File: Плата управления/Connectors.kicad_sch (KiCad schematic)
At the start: 10 parts, among them J1 A, J2 B, J3 C, J4 Conn_01x10, J5 Conn_01x03_Pin, J6 Conn_01x02, J7 Conn_01x10, J8 Conn_01x02, J9 Conn_01x04

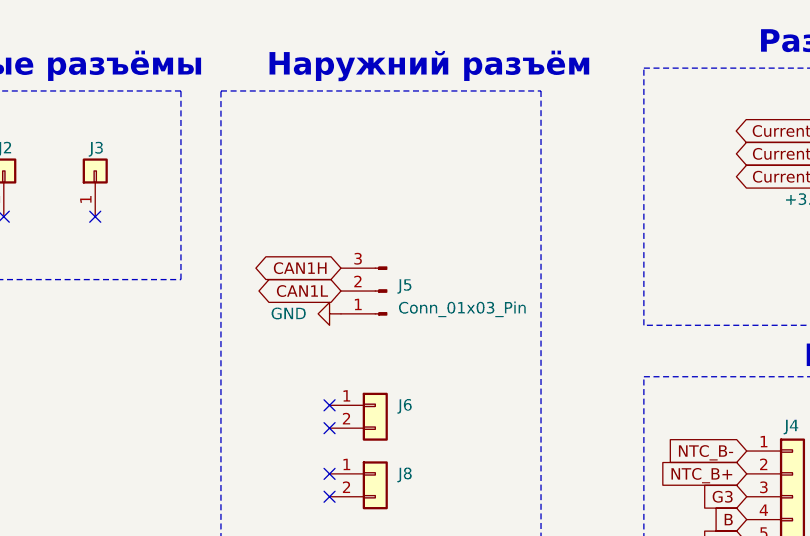
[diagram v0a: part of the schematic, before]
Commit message: Добавил модель плты
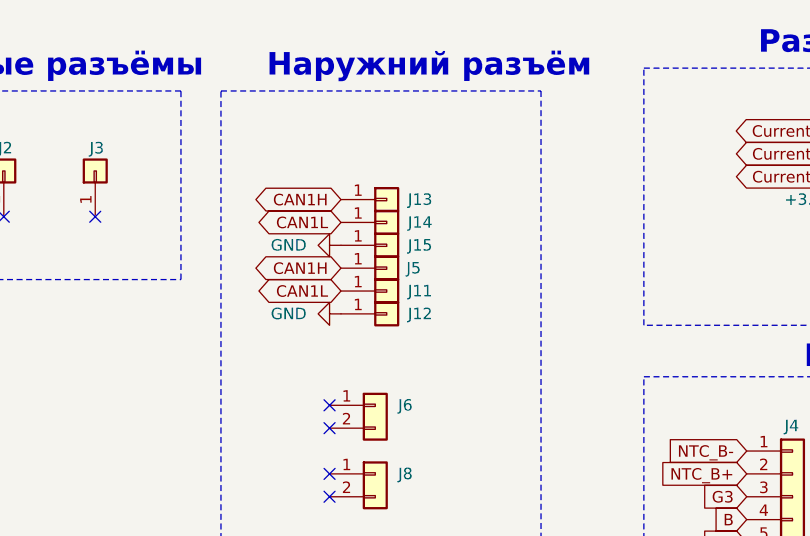
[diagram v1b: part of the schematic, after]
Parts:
- removed J5: Conn_01x03_Pin, Connector_PinHeader_2.54mm:PinHeader_1x03_P2.54mm_Vertical, symbol Connector:Conn_01x03_Pin
- added J11, J12, J13, J14, J15, J5: C, Connector_My:Wire_one, symbol Connector_Generic:Conn_01x01
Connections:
- net CAN1H: now also J13.1 (Pin_1), J5.1 (Pin_1)
- net CAN1L: now also J11.1 (Pin_1), J14.1 (Pin_1)
- net GND: now also J12.1 (Pin_1), J15.1 (Pin_1)
